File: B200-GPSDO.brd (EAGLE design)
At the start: 28.6 x 33.7 mm, 8 parts, among them U1 LEA-6T, U2 NC7SZ125, U3 NC7SZ125, U4 GPSDO

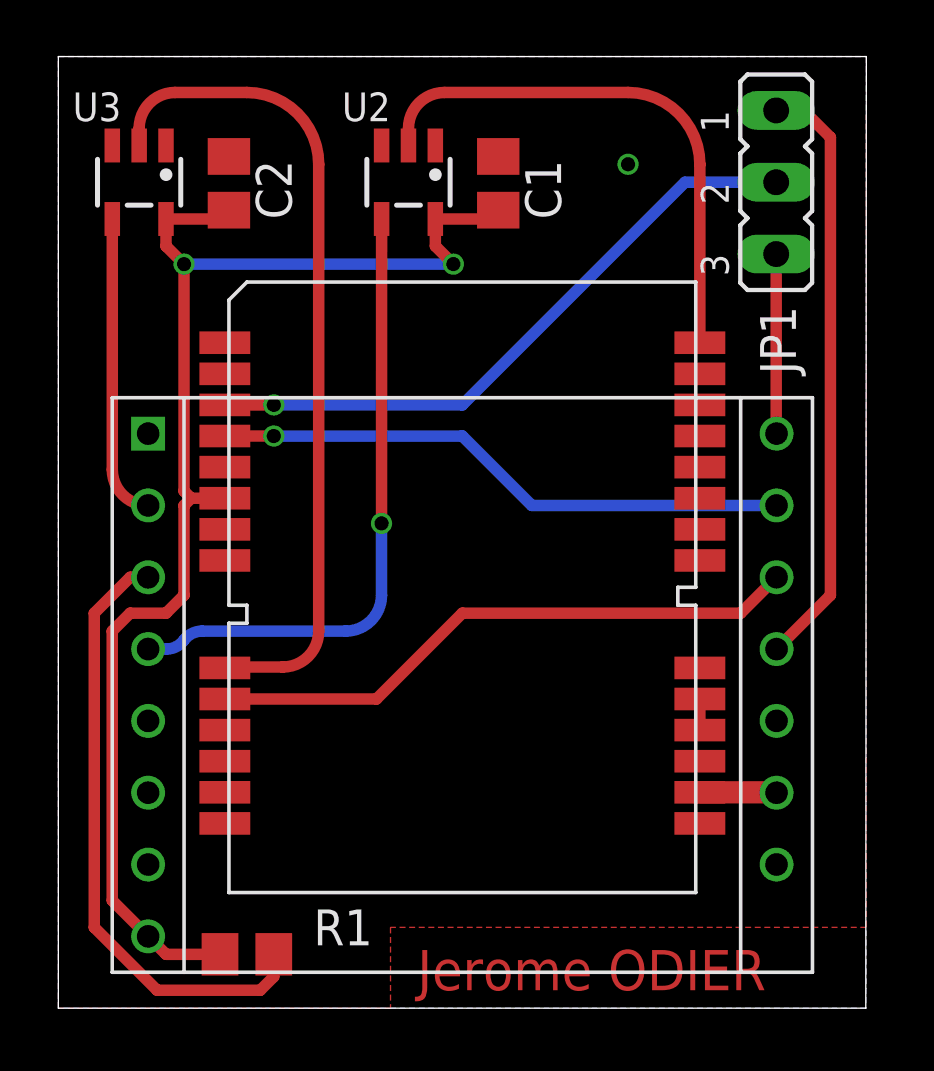
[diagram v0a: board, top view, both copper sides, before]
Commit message: update
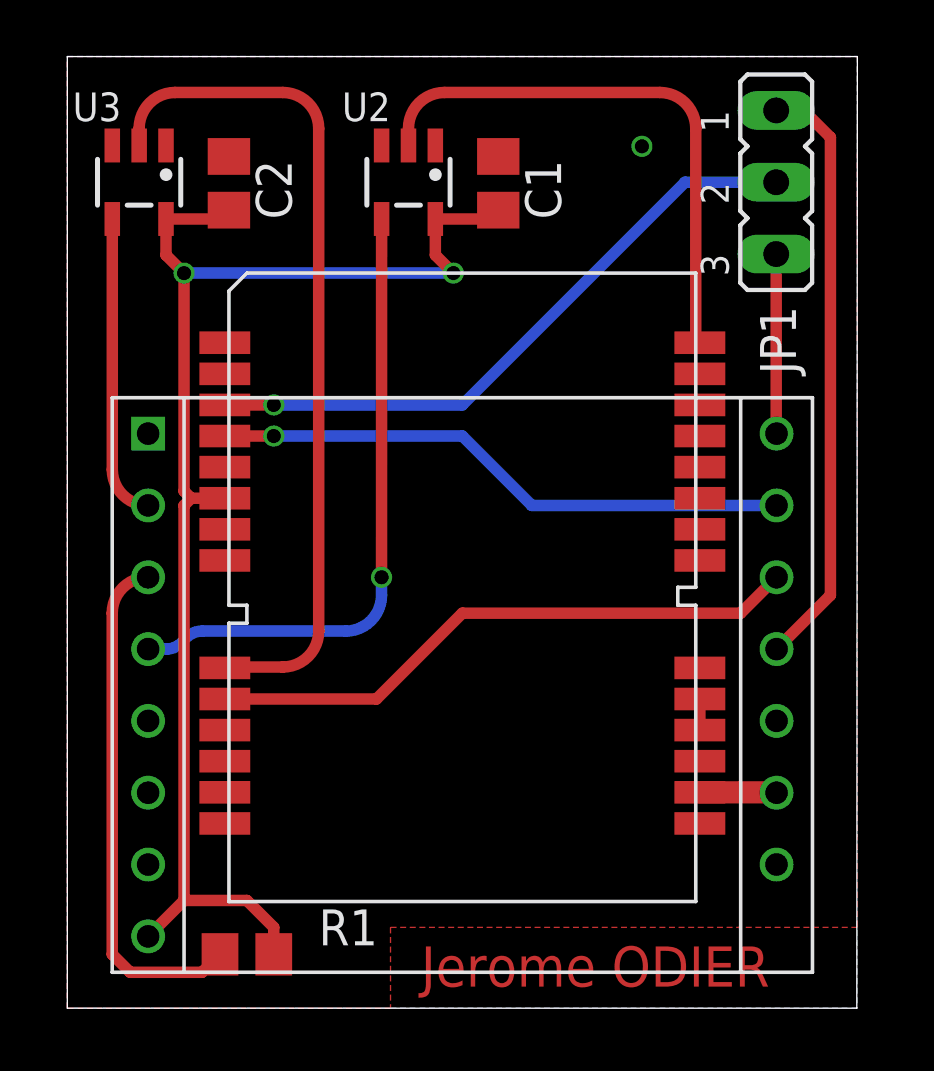
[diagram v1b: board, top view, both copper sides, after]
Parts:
- turned R1 to 0 degrees
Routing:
- net N$7: track 22.1 -> 18.2 mm
- net N$3: track 28.9 -> 29.6 mm
- net N$4: track 18.8 -> 19.5 mm
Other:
- board size 28.6 x 33.7 mm -> 27.9 x 33.7 mm
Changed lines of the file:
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@@
 <board>
 <plain>
-<wire x1="-0.3175" y1="0" x2="28.2375" y2="0" width="0" layer="20"/>
-<wire x1="28.2375" y1="0" x2="28.2575" y2="33.655" width="0" layer="20"/>
-<wire x1="28.2575" y1="33.655" x2="-0.3175" y2="33.655" width="0" layer="20"/>
-<wire x1="-0.3175" y1="33.655" x2="-0.3175" y2="0" width="0" layer="20"/>
-<text x="12.3825" y="0.635" size="1.4224" layer="1" font="vector" ratio="9">Jerome ODIER</text>
+<wire x1="0" y1="0" x2="27.92" y2="0" width="0" layer="20"/>
+<wire x1="27.92" y1="0" x2="27.94" y2="33.655" width="0" layer="20"/>
+<wire x1="27.94" y1="33.655" x2="0" y2="33.655" width="0" layer="20"/>
+<wire x1="0" y1="33.655" x2="0" y2="0" width="0" layer="20"/>
+<text x="12.5095" y="0.762" size="1.4224" layer="1" font="vector" ratio="9">Jerome ODIER</text>
 </plain>
 <attributes>
@@
 <attribute name="VALUE" x="20.7518" y="32.766" size="1.27" layer="27" ratio="10" rot="R270"/>
 </element>
-<element name="R1" library="rcl" package="R0805" value="1k" x="6.35" y="1.905" smashed="yes" rot="R180">
-<attribute name="NAME" x="10.795" y="3.4925" size="1.27" layer="25" rot="R180"/>
-<attribute name="VALUE" x="10.4775" y="1.5875" size="1.27" layer="27" rot="R180"/>
+<element name="R1" library="rcl" package="R0805" value="1k" x="6.35" y="1.905" smashed="yes">
+<attribute name="NAME" x="8.89" y="2.2225" size="1.27" layer="25"/>
+<attribute name="VALUE" x="8.89" y="0.3175" size="1.27" layer="27"/>
 </element>
 <element name="U1" library="B200-GPSDO" package="LEA" value="LEA-6T" x="13.97" y="14.8844" rot="R180"/>
@@
 <contactref element="R1" pad="2"/>
 <contactref element="U4" pad="8"/>
-<wire x1="2.8575" y1="2.54" x2="1.5875" y2="3.81" width="0.4064" layer="1"/>
-<wire x1="1.5875" y1="3.81" x2="1.5875" y2="13.335" width="0.4064" layer="1"/>
 <wire x1="5.57" y1="18.0344" x2="4.3819" y2="18.0344" width="0.4064" layer="1"/>
-<wire x1="4.3819" y1="18.0344" x2="4.1275" y2="17.78" width="0.4064" layer="1"/>
-<wire x1="4.1275" y1="17.78" x2="4.1275" y2="14.605" width="0.4064" layer="1"/>
-<wire x1="2.2225" y1="13.97" x2="3.4925" y2="13.97" width="0.4064" layer="1"/>
-<wire x1="3.4925" y1="13.97" x2="4.1275" y2="14.605" width="0.4064" layer="1"/>
-<via x="13.6525" y="26.3144" extent="1-16" drill="0.5"/>
+<via x="13.6525" y="25.9969" extent="1-16" drill="0.5"/>
 <wire x1="14.925" y1="27.9044" x2="15.24" y2="28.2219" width="0.4064" layer="1"/>
-<via x="4.1275" y="26.3144" extent="1-16" drill="0.5"/>
-<wire x1="4.1275" y1="26.3144" x2="13.6525" y2="26.3144" width="0.4064" layer="16"/>
-<wire x1="13.6525" y1="26.3144" x2="13.015" y2="26.9519" width="0.4064" layer="1"/>
-<wire x1="13.015" y1="26.9519" x2="13.015" y2="27.9099" width="0.4064" layer="1"/>
-<wire x1="4.1275" y1="26.3144" x2="3.49" y2="26.9519" width="0.4064" layer="1"/>
-<wire x1="3.49" y1="26.9519" x2="3.49" y2="27.9099" width="0.4064" layer="1"/>
-<wire x1="4.1275" y1="26.3144" x2="4.1275" y2="18.2888" width="0.4064" layer="1"/>
+<via x="4.1275" y="25.9969" extent="1-16" drill="0.5"/>
+<wire x1="4.1275" y1="25.9969" x2="13.6525" y2="25.9969" width="0.4064" layer="16"/>
+<wire x1="4.1275" y1="25.9969" x2="4.1275" y2="18.2888" width="0.4064" layer="1"/>
 <wire x1="4.1275" y1="18.2888" x2="4.3819" y2="18.0344" width="0.4064" layer="1"/>
-<wire x1="5.4" y1="1.905" x2="3.4925" y2="1.905" width="0.4064" layer="1"/>
-<wire x1="3.4925" y1="1.905" x2="2.8575" y2="2.54" width="0.4064" layer="1"/>
 <wire x1="13.015" y1="27.9099" x2="14.928" y2="27.9099" width="0.4064" layer="1"/>
 <wire x1="14.928" y1="27.9099" x2="15.24" y2="28.2219" width="0.4064" layer="1"/>
 <wire x1="3.49" y1="27.9099" x2="5.403" y2="27.9099" width="0.4064" layer="1"/>
 <wire x1="5.403" y1="27.9099" x2="5.715" y2="28.2219" width="0.4064" layer="1"/>
-<wire x1="1.5875" y1="13.335" x2="2.2225" y2="13.97" width="0.4064" layer="1"/>
+<wire x1="4.3819" y1="18.0344" x2="4.1275" y2="17.78" width="0.4064" layer="1"/>
+<wire x1="4.1275" y1="17.78" x2="4.1275" y2="3.81" width="0.4064" layer="1"/>
+<wire x1="4.1275" y1="3.81" x2="2.8575" y2="2.54" width="0.4064" layer="1"/>
+<wire x1="7.3" y1="1.905" x2="7.3" y2="2.86" width="0.4064" layer="1"/>
+<wire x1="7.3" y1="2.86" x2="6.35" y2="3.81" width="0.4064" layer="1"/>
+<wire x1="6.35" y1="3.81" x2="4.1275" y2="3.81" width="0.4064" layer="1"/>
+<wire x1="4.1275" y1="25.9969" x2="3.49" y2="26.6344" width="0.4064" layer="1"/>
+<wire x1="3.49" y1="26.6344" x2="3.49" y2="27.9099" width="0.4064" layer="1"/>
+<wire x1="13.6525" y1="25.9969" x2="13.015" y2="26.6344" width="0.4064" layer="1"/>
+<wire x1="13.015" y1="26.6344" x2="13.015" y2="27.9099" width="0.4064" layer="1"/>
 </signal>
 <signal name="RXD">
@@
 <contactref element="U3" pad="2"/>
 <contactref element="U1" pad="9"/>
-<wire x1="8.89" y1="29.845" x2="8.89" y2="13.335" width="0.4064" layer="1"/>
+<wire x1="8.89" y1="31.115" x2="8.89" y2="13.335" width="0.4064" layer="1"/>
 <wire x1="5.6006" y1="12.065" x2="5.57" y2="12.0344" width="0.4064" layer="1"/>
 <wire x1="5.6006" y1="12.065" x2="7.62" y2="12.065" width="0.4064" layer="1"/>
-<wire x1="3.81" y1="32.385" x2="6.35" y2="32.385" width="0.4064" layer="1"/>
+<wire x1="3.81" y1="32.385" x2="7.62" y2="32.385" width="0.4064" layer="1"/>
 <wire x1="2.54" y1="30.5101" x2="2.54" y2="31.115" width="0.4064" layer="1"/>
 <wire x1="2.54" y1="31.115" x2="3.81" y2="32.385" width="0.4064" layer="1" curve="-90"/>
 <wire x1="7.62" y1="12.065" x2="8.89" y2="13.335" width="0.4064" layer="1" curve="90"/>
-<wire x1="6.35" y1="32.385" x2="8.89" y2="29.845" width="0.4064" layer="1" curve="-90"/>
+<wire x1="7.62" y1="32.385" x2="8.89" y2="31.115" width="0.4064" layer="1" curve="-90"/>
 </signal>
 <signal name="N$4">
@@
 <wire x1="12.065" y1="30.5101" x2="12.065" y2="31.115" width="0.4064" layer="1"/>
 <wire x1="12.065" y1="31.115" x2="13.335" y2="32.385" width="0.4064" layer="1" curve="-90"/>
-<wire x1="22.37" y1="23.5344" x2="22.37" y2="29.845" width="0.4064" layer="1"/>
-<wire x1="19.83" y1="32.385" x2="13.335" y2="32.385" width="0.4064" layer="1"/>
-<wire x1="19.83" y1="32.385" x2="22.37" y2="29.845" width="0.4064" layer="1" curve="-90"/>
+<wire x1="20.955" y1="32.385" x2="13.335" y2="32.385" width="0.4064" layer="1"/>
+<wire x1="22.37" y1="23.5344" x2="22.225" y2="23.6794" width="0.4064" layer="1"/>
+<wire x1="22.225" y1="23.6794" x2="22.225" y2="31.115" width="0.4064" layer="1"/>
+<wire x1="20.955" y1="32.385" x2="22.225" y2="31.115" width="0.4064" layer="1" curve="-90"/>
 </signal>
 <signal name="RF_IN">
@@
 <contactref element="C2" pad="2"/>
 <polygon width="0.4064" layer="16">
-<vertex x="-0.3175" y="33.655"/>
-<vertex x="28.2575" y="33.655"/>
-<vertex x="28.2575" y="0"/>
-<vertex x="-0.3175" y="0"/>
+<vertex x="0" y="33.655"/>
+<vertex x="27.94" y="33.655"/>
+<vertex x="27.94" y="0"/>
+<vertex x="0" y="0"/>
 </polygon>
 <contactref element="U4" pad="1"/>
@@
 <contactref element="U4" pad="11"/>
 <polygon width="0.4064" layer="1">
-<vertex x="-0.3175" y="33.655"/>
-<vertex x="28.2575" y="33.655"/>
-<vertex x="28.2575" y="2.8575"/>
+<vertex x="0" y="33.655"/>
+<vertex x="27.94" y="33.655"/>
+<vertex x="27.94" y="2.8575"/>
 <vertex x="11.43" y="2.8575"/>
 <vertex x="11.43" y="0"/>
-<vertex x="-0.3175" y="0"/>
+<vertex x="0" y="0"/>
 </polygon>
-<via x="19.83" y="29.845" extent="1-16" drill="0.5"/>
+<via x="20.32" y="30.48" extent="1-16" drill="0.5"/>
 <contactref element="U1" pad="11"/>
 </signal>
@@
 <contactref element="U2" pad="4"/>
 <contactref element="U4" pad="4"/>
-<via x="11.1125" y="17.145" extent="1-16" drill="0.5"/>
+<via x="11.1125" y="15.24" extent="1-16" drill="0.5"/>
 <wire x1="3.4925" y1="12.7" x2="2.8575" y2="12.7" width="0.4064" layer="16"/>
 <wire x1="4.7625" y1="13.335" x2="9.8425" y2="13.335" width="0.4064" layer="16"/>
 <wire x1="3.4925" y1="12.7" x2="4.1275" y2="13.0175" width="0.4064" layer="16" curve="53.130102"/>
 <wire x1="4.1275" y1="13.0175" x2="4.7625" y2="13.335" width="0.4064" layer="16" curve="-53.130102"/>
-<wire x1="11.115" y1="27.9099" x2="11.1125" y2="17.145" width="0.4064" layer="1"/>
-<wire x1="11.1125" y1="17.145" x2="11.1125" y2="14.605" width="0.4064" layer="16"/>
+<wire x1="11.115" y1="27.9099" x2="11.1125" y2="15.24" width="0.4064" layer="1"/>
+<wire x1="11.1125" y1="15.24" x2="11.1125" y2="14.605" width="0.4064" layer="16"/>
 <wire x1="11.1125" y1="14.605" x2="9.8425" y2="13.335" width="0.4064" layer="16" curve="-90"/>
 </signal>
@@
 <contactref element="R1" pad="1"/>
 <contactref element="U4" pad="3"/>
-<wire x1="2.8575" y1="15.24" x2="2.2225" y2="15.24" width="0.4064" layer="1"/>
-<wire x1="2.2225" y1="15.24" x2="0.9525" y2="13.97" width="0.4064" layer="1"/>
-<wire x1="0.9525" y1="13.97" x2="0.9525" y2="2.8575" width="0.4064" layer="1"/>
-<wire x1="0.9525" y1="2.8575" x2="3.175" y2="0.635" width="0.4064" layer="1"/>
-<wire x1="3.175" y1="0.635" x2="6.823075" y2="0.635" width="0.4064" layer="1"/>
-<wire x1="7.3" y1="1.905" x2="7.3" y2="2.22" width="0.4064" layer="1"/>
-<wire x1="7.3" y1="1.905" x2="7.3" y2="1.111925" width="0.4064" layer="1"/>
-<wire x1="7.3" y1="1.111925" x2="6.823075" y2="0.635" width="0.4064" layer="1"/>
+<wire x1="1.5875" y1="13.97" x2="1.5875" y2="1.905" width="0.4064" layer="1"/>
+<wire x1="2.2225" y1="1.27" x2="1.5875" y2="1.905" width="0.4064" layer="1"/>
+<wire x1="2.8575" y1="15.24" x2="1.5875" y2="13.97" width="0.4064" layer="1" curve="90"/>
+<wire x1="2.2225" y1="1.27" x2="4.765" y2="1.27" width="0.4064" layer="1"/>
+<wire x1="4.765" y1="1.27" x2="5.4" y2="1.905" width="0.4064" layer="1"/>
 </signal>
 <signal name="N$8">
